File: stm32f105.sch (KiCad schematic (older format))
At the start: 0 parts

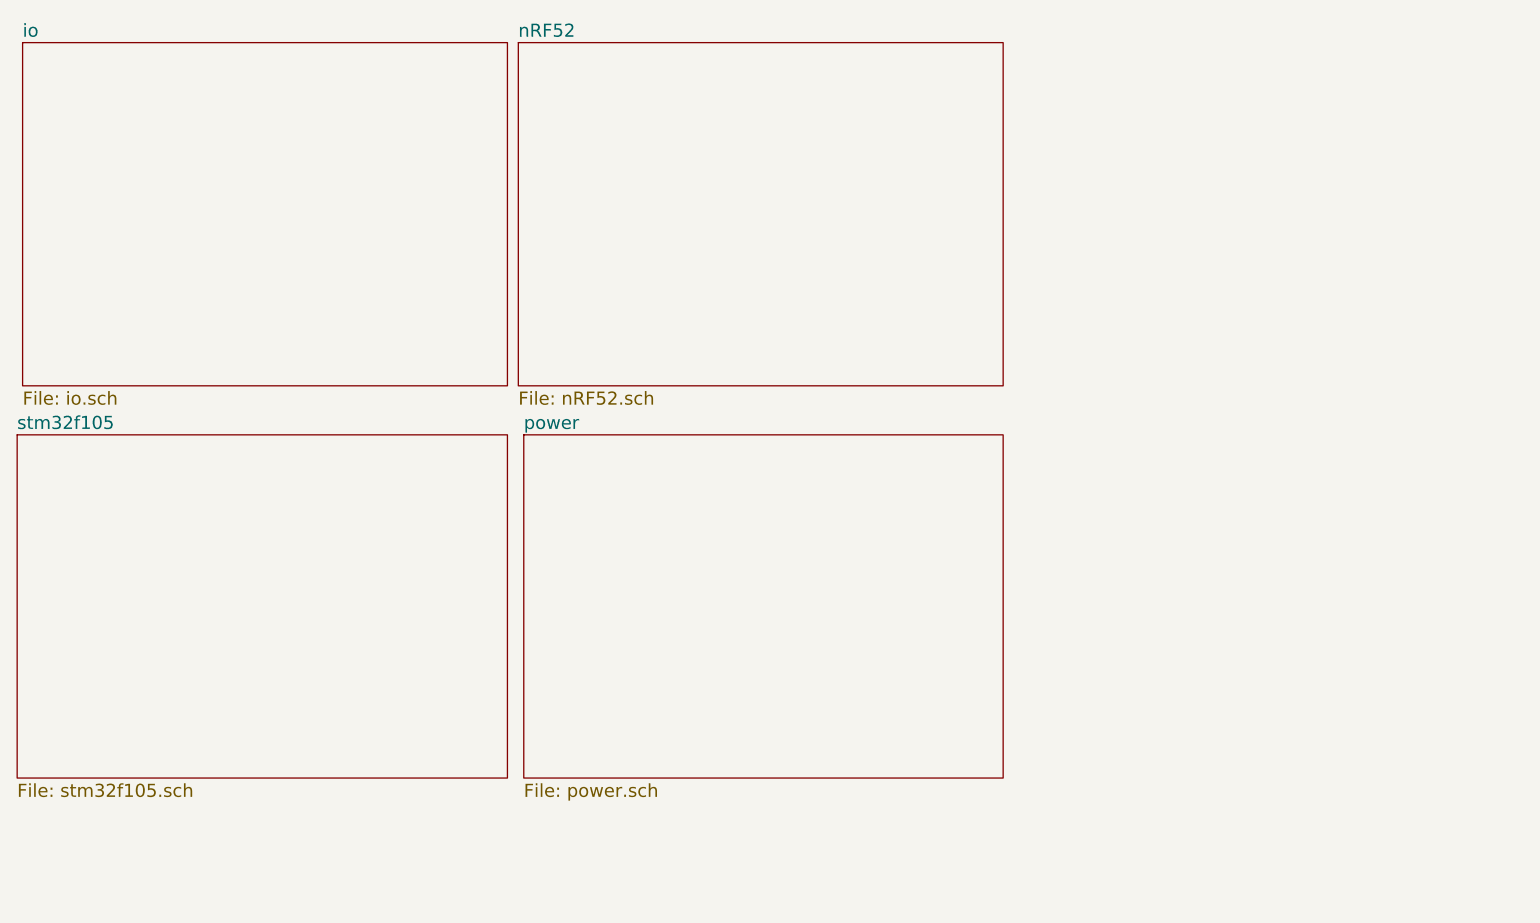
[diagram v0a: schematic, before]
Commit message: add schematics
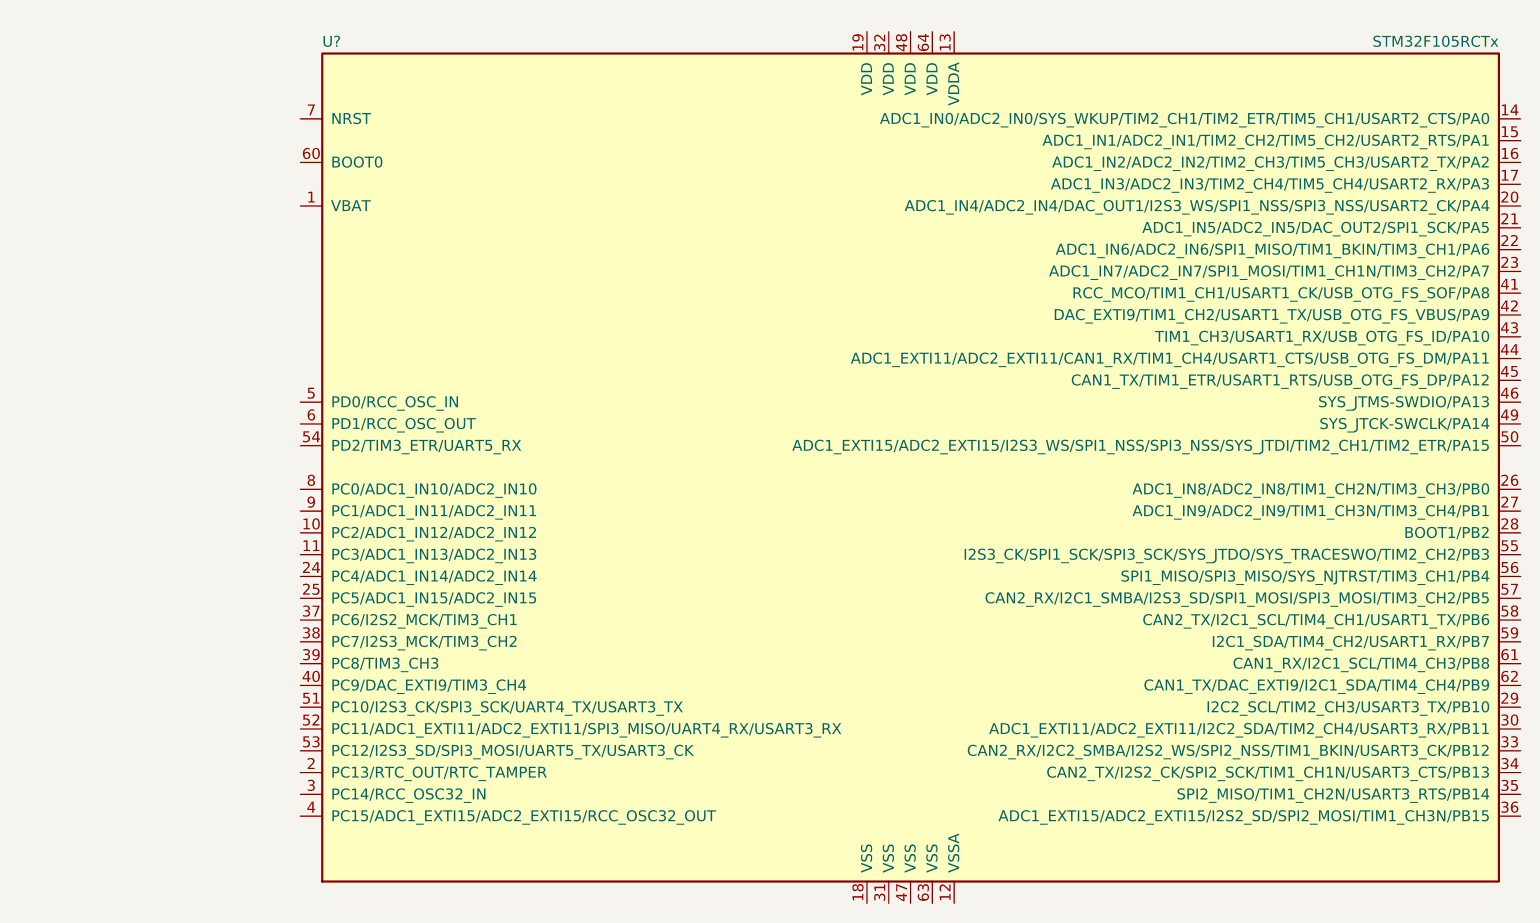
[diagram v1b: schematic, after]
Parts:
- added U?: STM32F105RCTx, LQFP64, symbol STM32F105RCTx
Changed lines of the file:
@@
 $Descr A4 11693 8268
 encoding utf-8
-Sheet 1 5
+Sheet 4 5
 Title ""
-Date "lun. 30 mars 2015"
+Date ""
 Rev ""
 Comp ""
@@
 Comment4 ""
 $EndDescr
-$Sheet
-S 1775 2025 2225 1575
-U 5A8ADEAA
-F0 "io" 60
-F1 "io.sch" 60
-$EndSheet
-$Sheet
-S 4050 2025 2225 1575
-U 5A8ADED7
-F0 "nRF52" 60
-F1 "nRF52.sch" 60
-$EndSheet
-$Sheet
-S 1750 3825 2250 1575
-U 5A8ADF8A
-F0 "stm32f105" 60
-F1 "stm32f105.sch" 60
-$EndSheet
-$Sheet
-S 4075 3825 2200 1575
-U 5A8ADFED
-F0 "power" 60
-F1 "power.sch" 60
-$EndSheet
+$Comp
+L STM32F105RCTx U?
+U 1 1 5A8AE7DC
+P 5850 3975
+F 0 "U?" H 3150 5900 50  0000 L BNN
+F 1 "STM32F105RCTx" H 8550 5900 50  0000 R BNN
+F 2 "LQFP64" H 8550 5850 50  0001 R TNN
+F 3 "" H 5850 3975 50  0001 C CNN
+	1    5850 3975
+	1    0    0    -1
+$EndComp
 $EndSCHEMATC
